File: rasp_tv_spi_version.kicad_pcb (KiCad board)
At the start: 2 copper layers, 120 x 60 mm, 16 parts, among them J1 Raspberry_Pi_2_3, J3 Conn_01x09, J4 AUODIO_IN, J5 SPEAKER, J6 AUDIO_OUT, J7 AUDIO_OUT, J8 Conn_01x02_Pin, J9 Raspberry_Pi_2_3, SW1 SW_Push_DPDT, U1 TFT_320x240, U2 PAM8302AAD

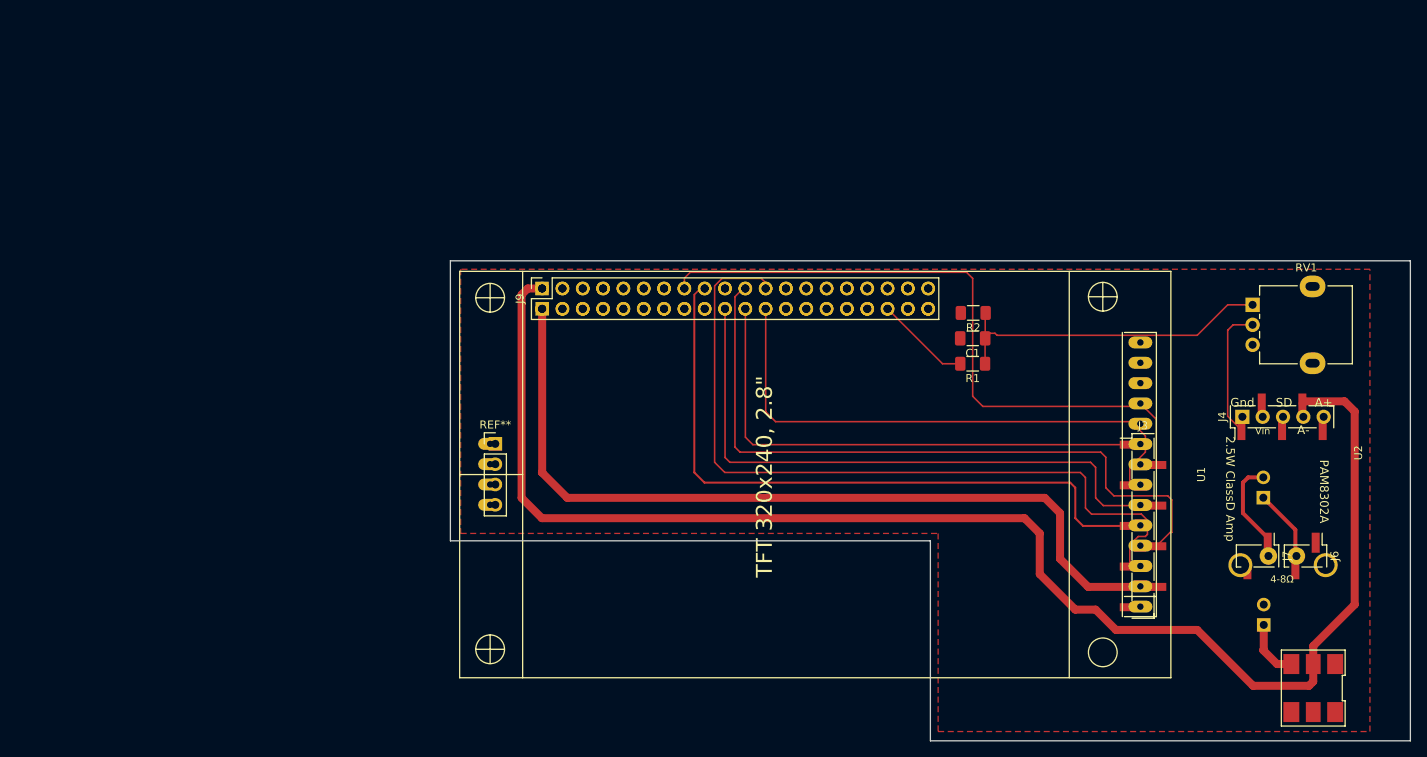
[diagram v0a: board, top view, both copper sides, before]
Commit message: release 2.8
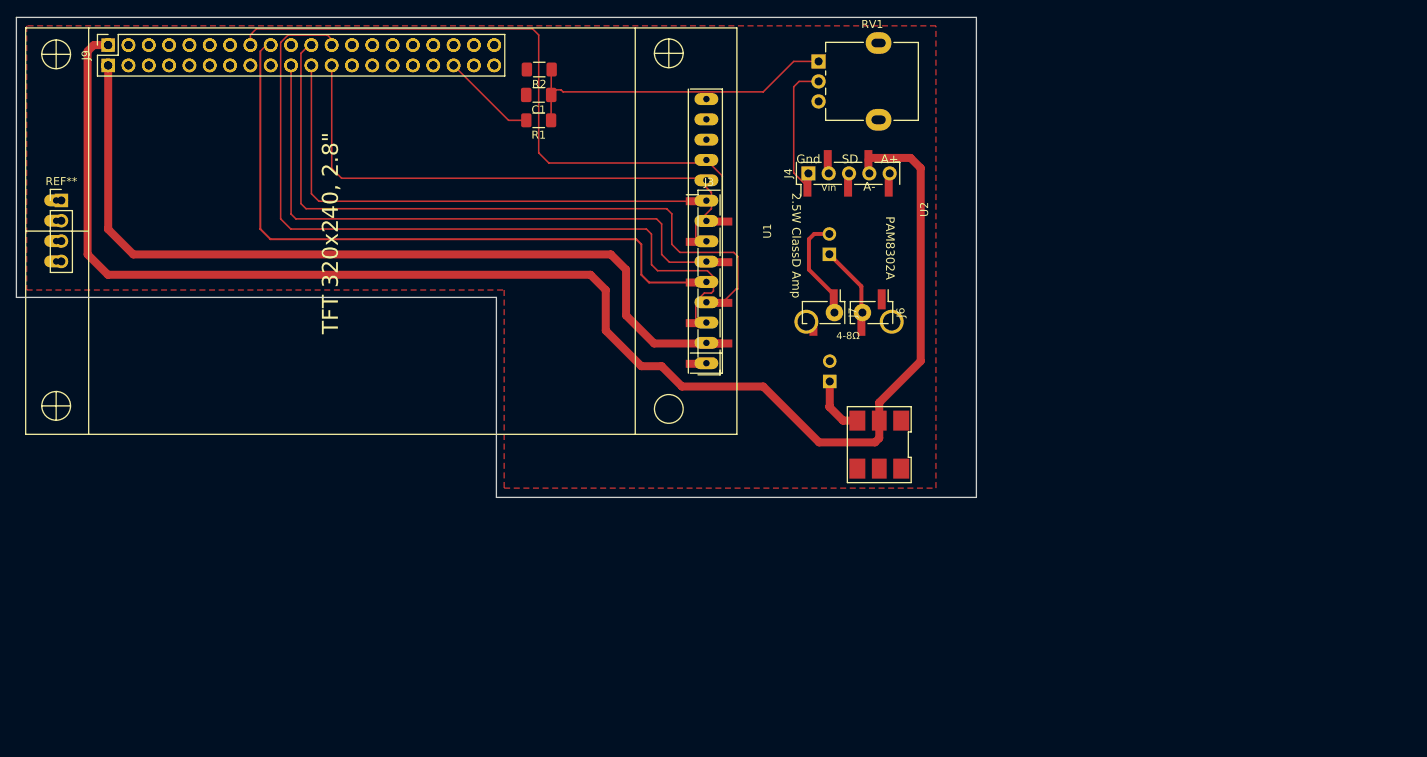
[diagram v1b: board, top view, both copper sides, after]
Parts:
- moved C1 62.2 mm to (91.0, 37.3)
- moved J3 62.2 mm to (112.3, 60.7)
- moved J4 62.2 mm to (129.7, 47.1)
- moved J5 62.2 mm to (127.4, 57.2)
- moved R1 62.2 mm to (91.0, 40.4)
- moved R2 62.2 mm to (91.1, 34.1)
- moved RV1 62.2 mm to (126.0, 33.1)
- moved U1 62.2 mm to (30.7, 76.1)
- moved U2 62.2 mm to (124.8, 47.1)
- moved J1 62.2 mm to (37.2, 33.6)
- moved J6 62.2 mm to (132.6, 64.5)
- moved J9 62.2 mm to (37.2, 31.0)
- moved REF** 62.2 mm to (31.4, 50.5)
- moved SW1 62.2 mm to (133.6, 81.0)
- moved J7 62.2 mm to (126.7, 64.5)
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
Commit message: ready for factory
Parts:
- removed the J4 at (129.7, 47.1)
- removed the J6 at (132.6, 64.5)
- removed the J7 at (126.7, 64.5)
- removed the J8 at (127.4, 73.1)
- removed REF**: PinHeader_1x04_P2.54mm_Vertical, Connector_PinHeader_2.54mm:PinHeader_1x04_P2.54mm_Vertical
- removed U2: PAM8302AAD, Module:PAM
- added 0.1u: C_Rect_L4.0mm_W2.5mm_P2.50mm, Capacitor_THT:C_Rect_L4.0mm_W2.5mm_P2.50mm, B.Cu at (247.6, 65.6)
- added 0.1u: C_Rect_L4.0mm_W2.5mm_P2.50mm, Capacitor_THT:C_Rect_L4.0mm_W2.5mm_P2.50mm, B.Cu at (224.6, 92.8)
- added 0.1u: C_Rect_L4.0mm_W2.5mm_P2.50mm, Capacitor_THT:C_Rect_L4.0mm_W2.5mm_P2.50mm, B.Cu at (249.5, 134.7)
- added 0.1u: C_Rect_L4.0mm_W2.5mm_P2.50mm, Capacitor_THT:C_Rect_L4.0mm_W2.5mm_P2.50mm, B.Cu at (97.5, 24.4)
- added 0.1u: C_Rect_L4.0mm_W2.5mm_P2.50mm, Capacitor_THT:C_Rect_L4.0mm_W2.5mm_P2.50mm, B.Cu at (122.4, 65.6)
- added 0.1u: C_Rect_L4.0mm_W2.5mm_P2.50mm, Capacitor_THT:C_Rect_L4.0mm_W2.5mm_P2.50mm, B.Cu at (222.6, 23.9)
- added 0.1uF: 0.1uF, Capacitor_SMD:C_1206_3216Metric_Pad1.33x1.80mm_HandSolder, F.Cu at (96.4, 26.3)
- added 0.1uF: 0.1uF, Capacitor_SMD:C_1206_3216Metric_Pad1.33x1.80mm_HandSolder, F.Cu at (125.2, 65.7)
- added 0.1uF: 0.1uF, Capacitor_SMD:C_1206_3216Metric_Pad1.33x1.80mm_HandSolder, F.Cu at (250.4, 65.7)
- added 0.1uF: 0.1uF, Capacitor_SMD:C_1206_3216Metric_Pad1.33x1.80mm_HandSolder, F.Cu at (252.3, 134.8)
- added 0R: R_1206_3216Metric, Resistor_SMD:R_1206_3216Metric, F.Cu at (186.5, 25.6)
- added 0R: R_1206_3216Metric, Resistor_SMD:R_1206_3216Metric, F.Cu at (188.5, 94.6)
- added 0R: R_1206_3216Metric, Resistor_SMD:R_1206_3216Metric, F.Cu at (237.0, 59.0)
- added 0R: R_1206_3216Metric, Resistor_SMD:R_1206_3216Metric, F.Cu at (239.3, 127.9)
- added 0R: , Resistor_SMD:R_1206_3216Metric, F.Cu at (61.5, 25.6)
- added 0R: , Resistor_SMD:R_1206_3216Metric, F.Cu at (111.6, 58.9)
- added 100R: R_Axial_DIN0204_L3.6mm_D1.6mm_P5.08mm_Horizontal, Resistor_THT:R_Axial_DIN0204_L3.6mm_D1.6mm_P5.08mm_Horizontal, B.Cu at (223.8, 30.9)
- added 100R: R_Axial_DIN0204_L3.6mm_D1.6mm_P5.08mm_Horizontal, Resistor_THT:R_Axial_DIN0204_L3.6mm_D1.6mm_P5.08mm_Horizontal, B.Cu at (225.8, 99.8)
- added 100R: R_Axial_DIN0204_L3.6mm_D1.6mm_P5.08mm_Horizontal, Resistor_THT:R_Axial_DIN0204_L3.6mm_D1.6mm_P5.08mm_Horizontal, B.Cu at (98.8, 31.0)
- added 100uF: CP_Radial_D5.0mm_P2.50mm, Capacitor_THT:CP_Radial_D5.0mm_P2.50mm, B.Cu at (249.9, 61.8)
- added 100uF: CP_Radial_D5.0mm_P2.50mm, Capacitor_THT:CP_Radial_D5.0mm_P2.50mm, B.Cu at (251.8, 130.9)
- added 100uF: CP_Radial_D5.0mm_P2.50mm, Capacitor_THT:CP_Radial_D5.0mm_P2.50mm, B.Cu at (124.7, 61.8)
- added 1K: 1K, Potentiometer_THT:Potentiometer_Alpha_RD901F-40-00D_Single_Vertical, F.Cu at (124.3, 22.1)
- added 220R: , Resistor_SMD:R_1206_3216Metric_Pad1.30x1.75mm_HandSolder, F.Cu at (96.2, 21.6)
- added 220R: 220R, Resistor_THT:R_Axial_DIN0204_L3.6mm_D1.6mm_P5.08mm_Horizontal, B.Cu at (98.8, 19.8)
- added 220R: 220R, Resistor_THT:R_Axial_DIN0204_L3.6mm_D1.6mm_P5.08mm_Horizontal, B.Cu at (225.8, 88.6)
- added 220R: 220R, Resistor_THT:R_Axial_DIN0204_L3.6mm_D1.6mm_P5.08mm_Horizontal, B.Cu at (223.8, 19.7)
- added ?: , , F.Cu at (251.8, 130.9)
- added ?: , , F.Cu at (247.6, 65.6)
- added ?: , , F.Cu at (252.3, 136.4)
- added ?: , , F.Cu at (247.6, 68.1)
- added ?: , , F.Cu at (224.6, 92.8)
- added C1: 0.1uF, Capacitor_SMD:C_1206_3216Metric_Pad1.33x1.80mm_HandSolder, F.Cu at (223.4, 95.3)
- added HOLD: PinHeader_1x02_P2.54mm_Vertical_SMD_Pin1Right, Connector_PinHeader_2.54mm:PinHeader_1x02_P2.54mm_Vertical_SMD_Pin1Right, F.Cu at (160.4, 109.8)
- added HOLD: HOLD, Connector_PinHeader_2.54mm:PinHeader_1x02_P2.54mm_Vertical_SMD_Pin1Right, F.Cu at (161.7, 40.8)
- added HOLD: PinHeader_1x02_P2.54mm_Vertical_SMD_Pin1Right, Connector_PinHeader_2.54mm:PinHeader_1x02_P2.54mm_Vertical_SMD_Pin1Right, F.Cu at (22.9, 40.8)
- added J3: Conn_01x09, Connector_PinHeader_2.54mm:PinHeader_1x09_P2.54mm_Vertical_SMD_Pin1Left, F.Cu at (117.7, 49.7)
- added J4: Conn_01x05_Pin, Connector_PinHeader_2.54mm:PinHeader_1x05_P2.54mm_Vertical, B.Cu at (249.7, 34.7)
- added J4: Conn_01x05_Pin, Connector_PinHeader_2.54mm:PinHeader_1x05_P2.54mm_Vertical, B.Cu at (124.7, 34.7)
- added J6: OUT1, Connector_PinHeader_2.54mm:PinHeader_1x01_P2.54mm_Vertical, B.Cu at (128.1, 52.1)
- added J6: OUT1, Connector_PinHeader_2.54mm:PinHeader_1x01_P2.54mm_Vertical, B.Cu at (255.1, 121.1)
- added J6: OUT1, Connector_PinHeader_2.54mm:PinHeader_1x01_P2.54mm_Vertical, B.Cu at (253.1, 52.1)
- added J7: OUT2, Connector_PinHeader_2.54mm:PinHeader_1x01_P2.54mm_Vertical, B.Cu at (131.6, 52.1)
- added J7: OUT2, Connector_PinHeader_2.54mm:PinHeader_1x01_P2.54mm_Vertical, B.Cu at (256.6, 52.1)
- added J7: OUT2, Connector_PinHeader_2.54mm:PinHeader_1x01_P2.54mm_Vertical, B.Cu at (258.6, 121.1)
- added J8: Conn_01x02_Pin, Connector_Wire:SolderWire-0.1sqmm_1x02_P3.6mm_D0.4mm_OD1mm, F.Cu at (260.9, 57.0)
- added J8: Conn_01x02_Pin, Connector_Wire:SolderWire-0.1sqmm_1x02_P3.6mm_D0.4mm_OD1mm, F.Cu at (262.9, 126.0)
- added J8: Conn_01x02_Pin, Connector_Wire:SolderWire-0.1sqmm_1x02_P3.6mm_D0.4mm_OD1mm, F.Cu at (135.9, 57.0)
- added J9: Raspberry_Pi_2_3, Connector_PinSocket_2.54mm:PinSocket_2x20_P2.54mm_Vertical, F.Cu at (42.6, 20.0)
- added J9: Raspberry_Pi_2_3, Connector_PinSocket_2.54mm:PinSocket_2x20_P2.54mm_Vertical, F.Cu at (169.6, 89.0)
- added PAM8302: PAM, Module:PAM, B.Cu at (259.9, 34.7)
- added PAM8302: PAM, Module:PAM, B.Cu at (262.0, 103.7)
- added PAM8302: PAM, Module:PAM, B.Cu at (134.9, 34.7)
- added PAM8302: Conn_01x05_Pin, Connector_PinHeader_2.54mm:PinHeader_1x05_P2.54mm_Vertical, B.Cu at (251.7, 103.7)
- added R1: 100E, Resistor_SMD:R_1206_3216Metric_Pad1.30x1.75mm_HandSolder, F.Cu at (223.4, 98.4)
- added R1: 100R, Resistor_SMD:R_1206_3216Metric_Pad1.30x1.75mm_HandSolder, F.Cu at (96.4, 29.4)
- added R2: 220E, Resistor_SMD:R_1206_3216Metric_Pad1.30x1.75mm_HandSolder, F.Cu at (223.4, 90.6)
- added RV1: 1K, Potentiometer_THT:Potentiometer_Alpha_RD901F-40-00D_Single_Vertical, F.Cu at (251.3, 91.1)
- added Raspberry_Pi_ZERO: Raspberry_Pi_2_3, Connector_PinSocket_2.54mm:PinSocket_2x20_P2.54mm_Vertical, B.Cu at (42.6, 22.6)
- added Raspberry_Pi_ZERO: Raspberry_Pi_2_3, Connector_PinSocket_2.54mm:PinSocket_2x20_P2.54mm_Vertical, B.Cu at (169.6, 91.6)
- added SPEAKER: SPEAKER, Connector_Hirose:Hirose_DF3EA-02P-2V_1x02-1MP_P2.00mm_Vertical, F.Cu at (253.2, 43.3)
- added SPEAKER: SPEAKER, Connector_Hirose:Hirose_DF3EA-02P-2V_1x02-1MP_P2.00mm_Vertical, F.Cu at (128.2, 43.3)
- added SW: SW_Push_DPDT, Button_Switch_THT:SW_DPDT_XLX, F.Cu at (131.8, 64.0)
- added SW: SW_Push_DPDT, Button_Switch_THT:SW_DPDT_XLX, F.Cu at (258.8, 133.0)
- added TFT320x240,3.2": Conn_01x09, Connector_PinHeader_2.54mm:PinHeader_1x09_P2.54mm_Vertical_SMD_Pin1Left, F.Cu at (244.7, 118.7)
- added U1: TFT_320x240, Display:TFT-320x240, F.Cu at (163.3, 134.3)
- added U1: TFT_320x240, Display:TFT-320x240, F.Cu at (35.9, 65.3)
- J5: footprint Connector_PinHeader_2.54mm:PinHeader_1x02_P2.54mm_Horizontal -> Connector_Hirose:Hirose_DF3EA-02P-2V_1x02-1MP_P2.00mm_Vertical; moved to F.Cu
- Raspberry_Pi_ZERO: renamed from J1; value Raspberry_Pi_2_3 -> Raspberry_Pi_ZERO
- SW: renamed from SW1; value SW_Push_DPDT -> SW
- moved J5 139.2 mm to (255.2, 112.3), turned to 90 degrees
- moved R2 130.9 mm to (221.4, 21.7)
- moved J9 130.9 mm to (167.6, 20.0)
- moved R1 130.8 mm to (221.4, 29.4)
- moved TFT320x240,2.8" 130.8 mm to (242.7, 49.7)
- moved C1 130.8 mm to (221.4, 26.3)
- moved Raspberry_Pi_ZERO 130.8 mm to (167.6, 22.6)
- moved U1 130.7 mm to (160.9, 65.3)
- moved SW 124.4 mm to (256.8, 64.0), turned to 0 degrees
- moved 1K 123.8 mm to (249.3, 22.1)
- renumbered RV1 to 1K, J3 to TFT320x240,2.8"
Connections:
- 1K pad : (no net) -> GND
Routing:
- net +5V: track 183.3 -> 511.5 mm
- net BACKLIGHT_23_GPIO: track 82.5 -> 255.0 mm
- net CS_8_GPIO: track 96.3 -> 268.0 mm
- net RESET_25_GPIO: track 86.8 -> 257.6 mm
- net DC_24_GPIO: track 83.3 -> 227.6 mm
- net +3.3V: track 106.5 -> 249.3 mm
- net MOSI_0_10_GPIO: track 77.3 -> 211.9 mm
- net SCK_0_11_GPIO: track 68.6 -> 196.7 mm
- net MISO_0_09_GPIO: track 64.5 -> 173.1 mm
- net Net-(C1-Pad1): track 42.2 -> 121.3 mm
- net Net-(J5-Pin_2): track 11.6 -> 58.3 mm
- net Net-(J8-Pin_2): track 0.01 -> 32.6 mm
- net Net-(J8-Pin_1): track 7.62 -> 38.4 mm
- net PWM_19_GPIO: track 11.9 -> 41.5 mm
- net AUDIO_IN: track 16.6 -> 39.7 mm
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- added copper zone on F.Cu, net +5V
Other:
- board size 120 x 60 mm -> 247 x 123 mm
- board text added: "+"
- board text added: "-"
- board text added: "PAM8302A"
